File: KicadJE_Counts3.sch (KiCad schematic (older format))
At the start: 78 parts, among them J301 ClockOut, J303 ClockIn, J304 Out0, J305 Out1, J306 Out2, J307 Out3, J308 Out4, J309 Out5, J310 Out6, J311 Out7, J312 Out8, J313 Out9, J314 Reset, P301 HEADER_2x5_Doepfer, SW301 Run

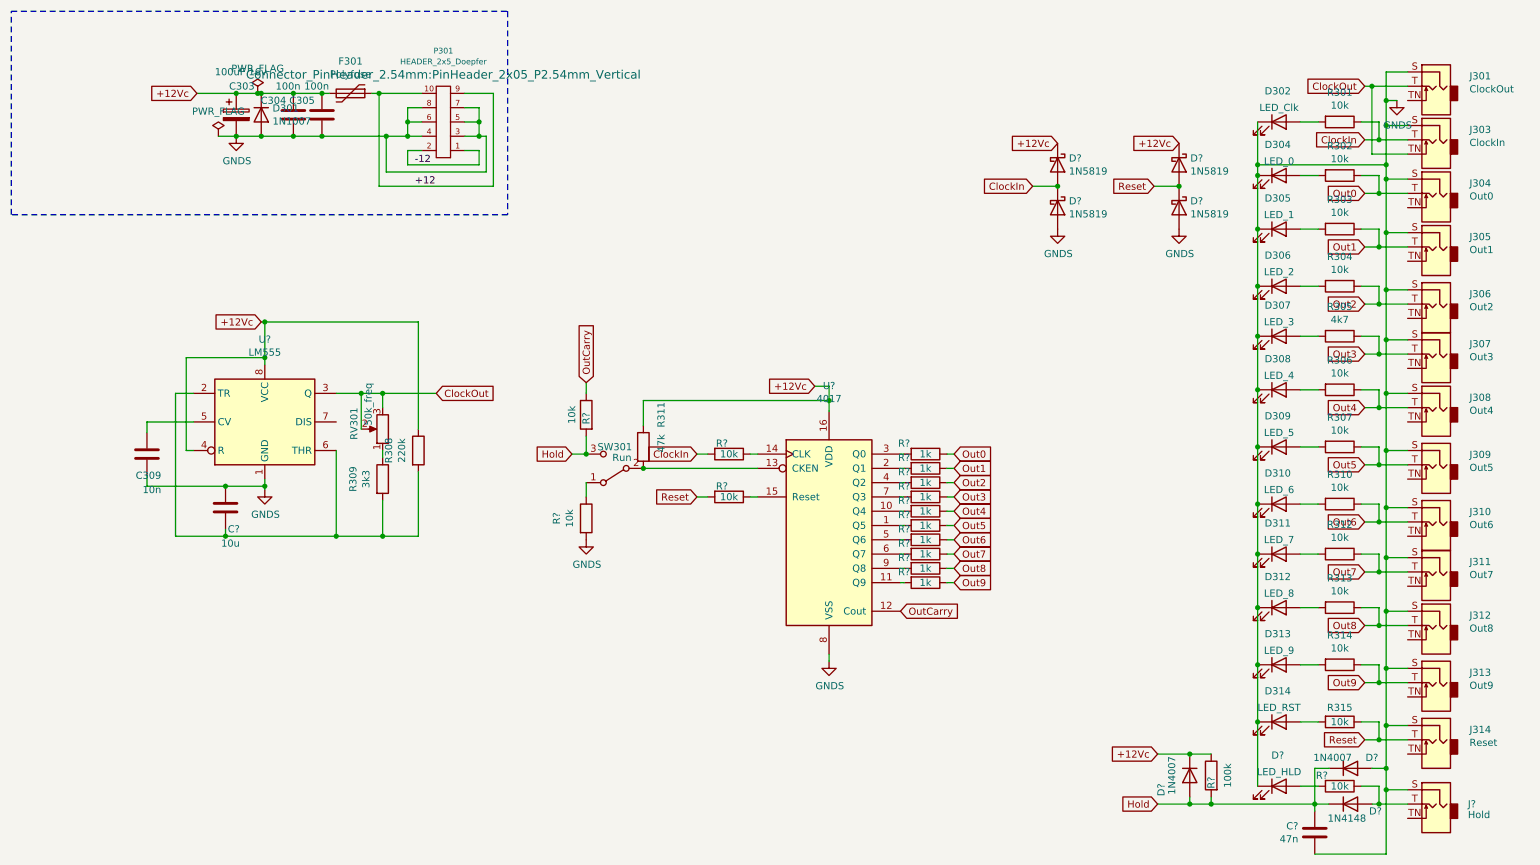
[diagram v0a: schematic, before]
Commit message: sch updates
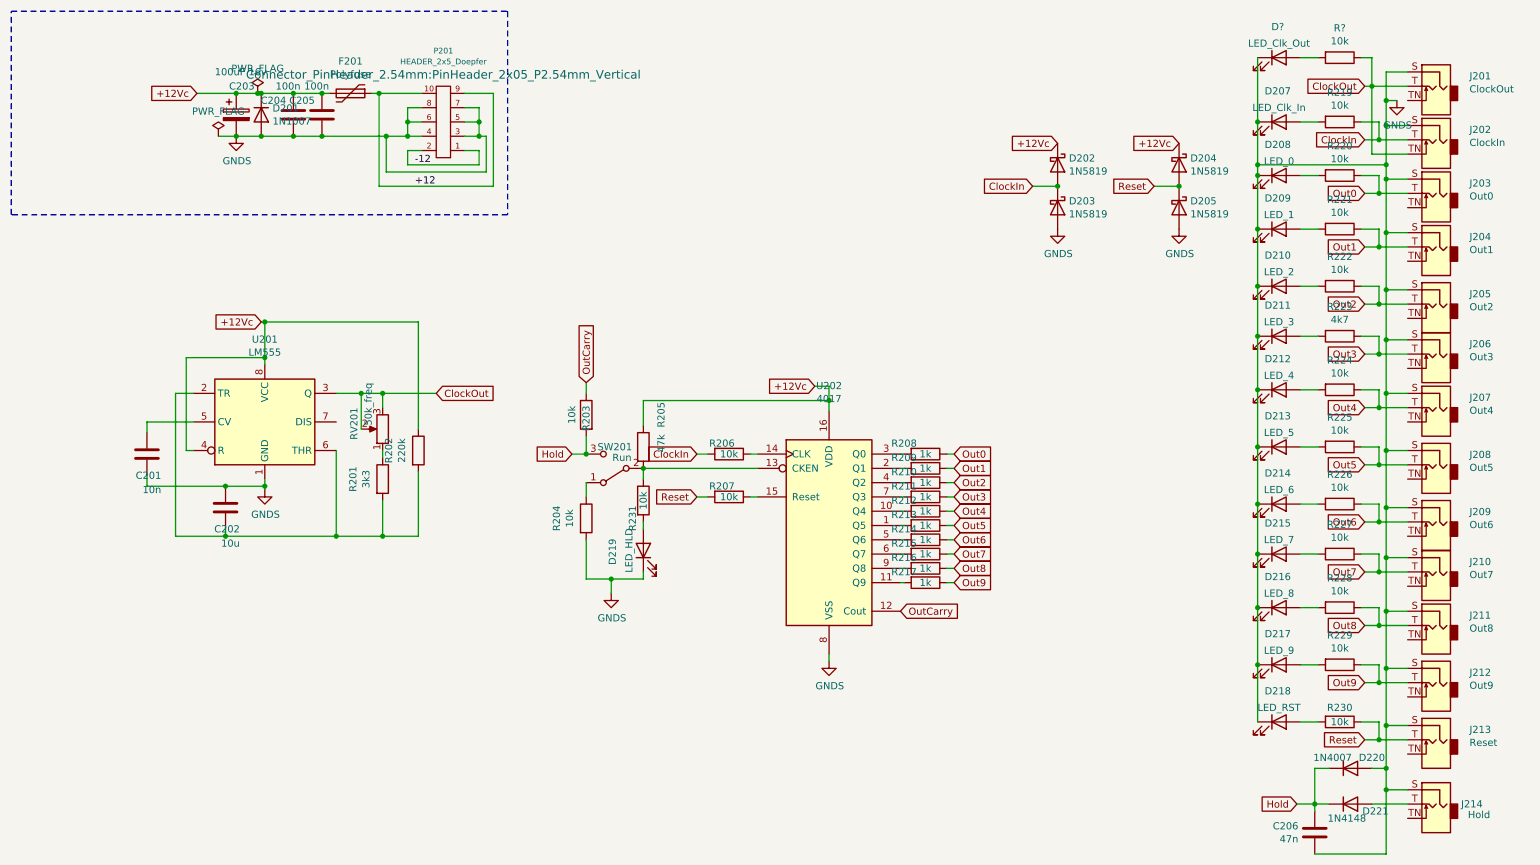
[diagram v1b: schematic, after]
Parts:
- removed D?: 1N4007, Diode_SMD:D_MiniMELF, symbol Diode:LL4148
- removed R?: 100k, AJ:R_0805_AJ, symbol Device:R
- added D?: LED_Clk_Out, LED_THT:LED_D3.0mm, symbol Device:LED
- added R?: 10k, Resistor_SMD:R_0805_2012Metric_Pad1.15x1.40mm_HandSolder, symbol Device:R
- D207: renamed from D302; value LED_Clk -> LED_Clk_In
- J214: renamed from J?; footprint Connector_Audio:Jack_3.5mm_Ledino_KB3SPRS_Horizontal -> AJ-Dropbox-Kicad:PJ301SM
- gave numbers to parts that had none: 26
- renumbered C309 to C201, C303 to C203, C304 to C204, C305 to C205, D301 to D201, D304 to D208, D305 to D209, D306 to D210, D307 to D211, D308 to D212, D309 to D213, D310 to D214, D311 to D215, D312 to D216, D313 to D217, D314 to D218, F301 to F201, J301 to J201, J303 to J202, J304 to J203, J305 to J204, J306 to J205, J307 to J206, J308 to J207, J309 to J208, J310 to J209, J311 to J210, J312 to J211, J313 to J212, J314 to J213, P301 to P201, R309 to R201, R308 to R202, R311 to R205, R301 to R219, R302 to R220, R303 to R221, R304 to R222, R305 to R223, R306 to R224, R307 to R225, R310 to R226, R312 to R227, R313 to R228, R314 to R229, R315 to R230, RV301 to RV201, SW301 to SW201
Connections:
- net ClockOut: now also R?.1
- net GNDS: now also D?.1 (K)
- net at R205.2, SW201.2 (B), U202.13 (CKEN): now also R231.1
- net at D221.2 (A), J214.T: no longer R231.1
- new net: D?.2 (A), R?.2
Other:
- moved on the sheet: D219, R231
